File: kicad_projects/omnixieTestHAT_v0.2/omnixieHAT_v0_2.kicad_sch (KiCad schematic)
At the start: 10 parts, among them J1 IL-WX-16PB-VF-B-E1000E, J2 Conn_02x08_Counter_Clockwise

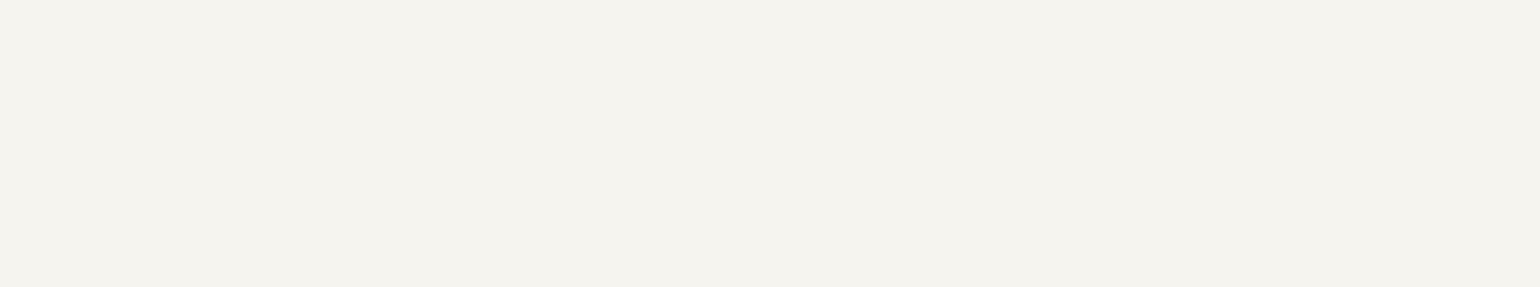
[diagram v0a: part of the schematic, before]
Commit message: redlines almost done, new layout commencing
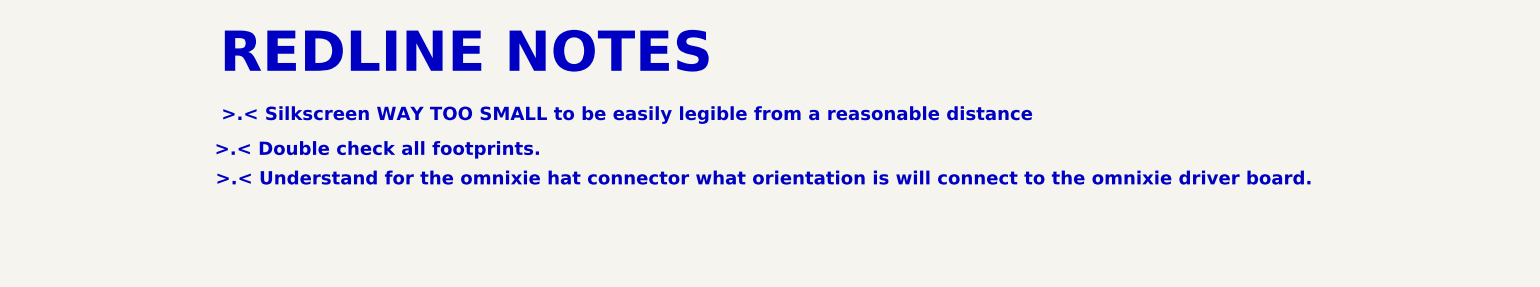
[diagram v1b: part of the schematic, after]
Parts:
- N1, N2, N3, N5, N6, N7: value ~ -> (none)
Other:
- note added: ">.< Double check all footprints."
- note added: ">.< Silkscreen WAY TOO SMALL to be easily legible from a reasonable distance"
- note added: ">.< Understand for the omnixie hat connector what orientation is will connect to the omnixie driver board."
- note added: "REDLINE NOTES"
